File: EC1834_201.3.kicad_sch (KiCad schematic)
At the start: 72 parts

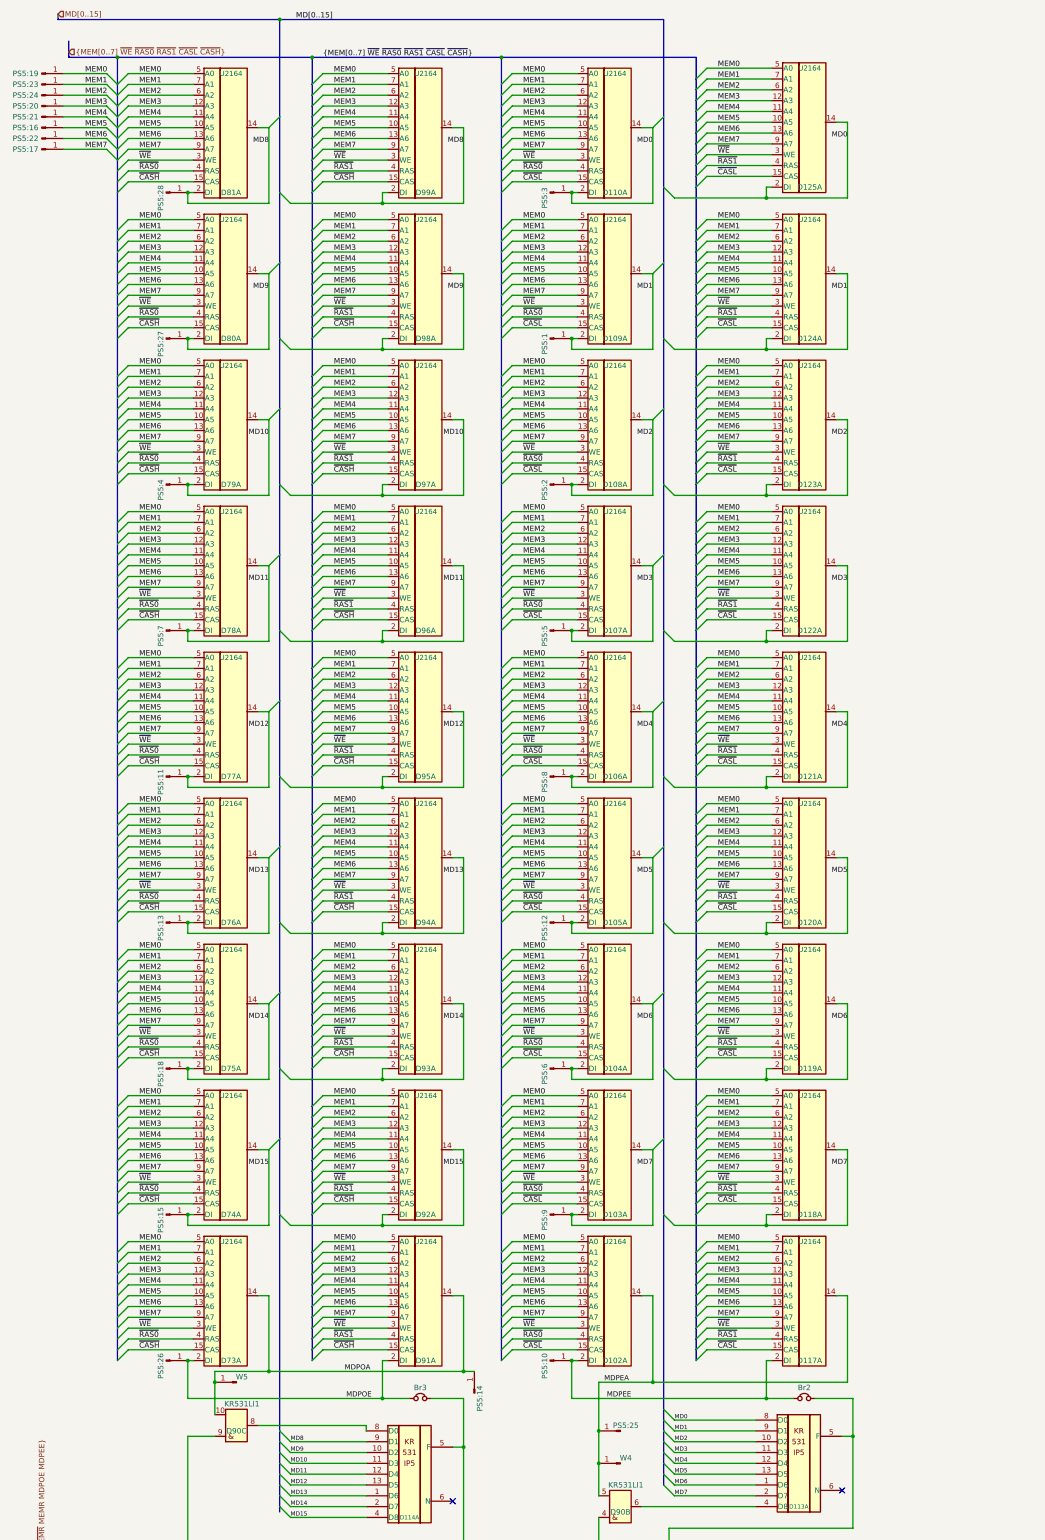
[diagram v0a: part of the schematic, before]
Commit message: Completed PCB layout Changed PS5
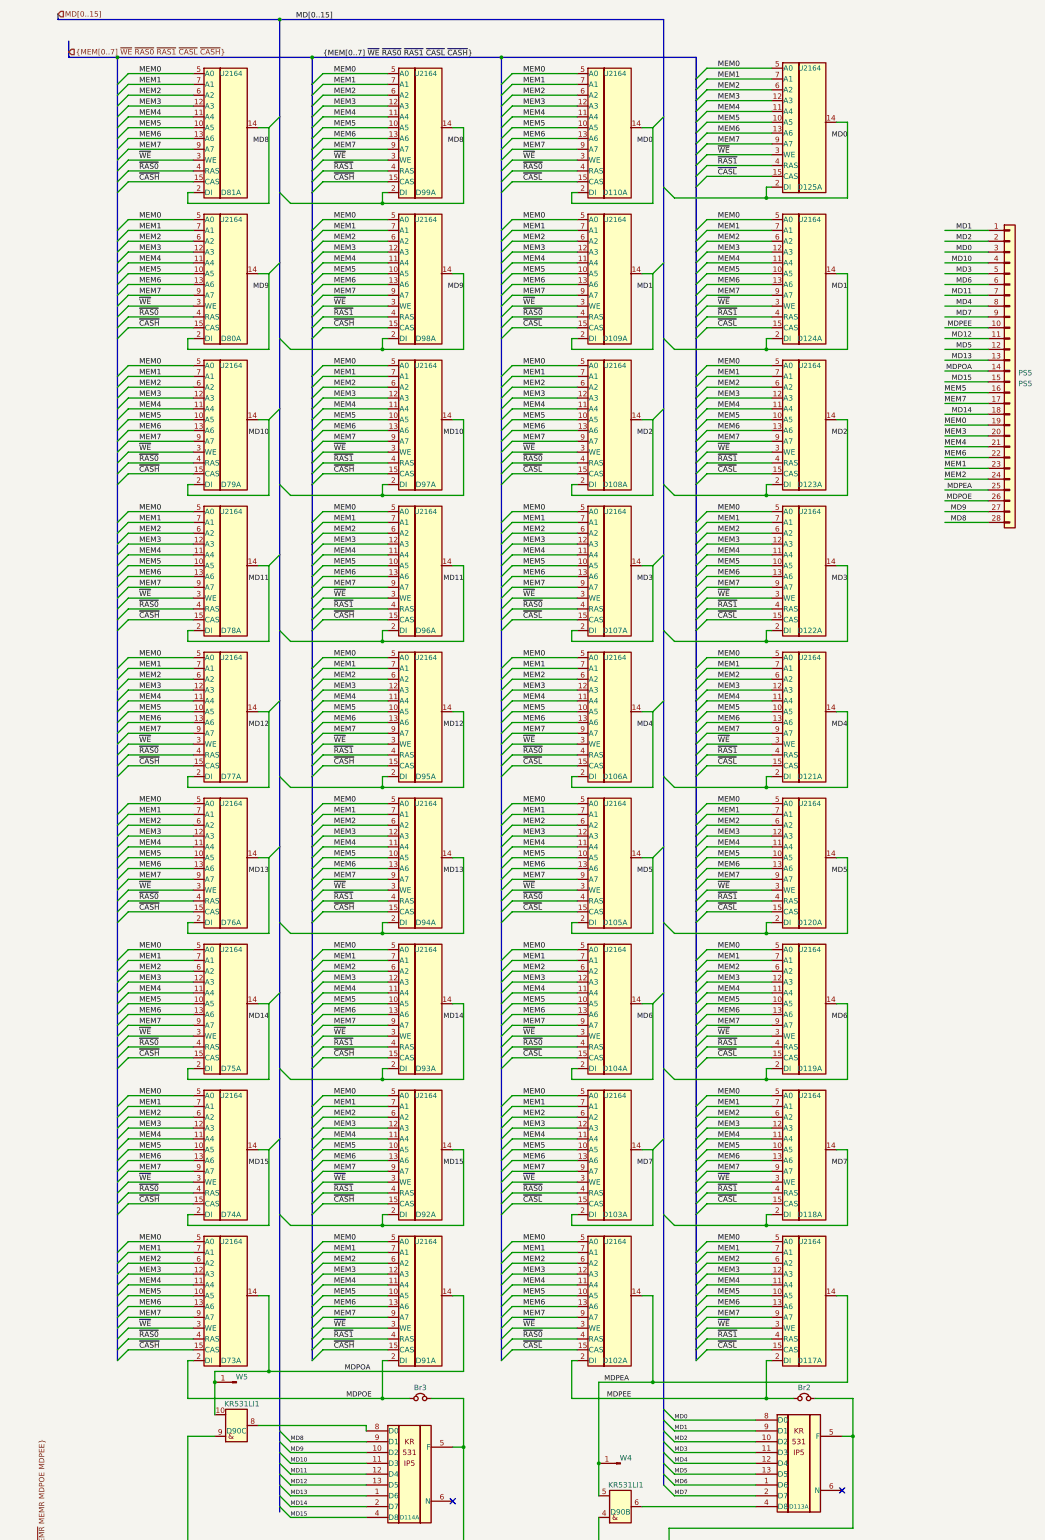
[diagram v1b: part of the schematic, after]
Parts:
- removed PS5:1, PS5:10, PS5:11, PS5:12, PS5:13, PS5:14, PS5:15, PS5:16, PS5:17, PS5:18, PS5:19, PS5:2, PS5:20, PS5:21, PS5:22, PS5:23, PS5:24, PS5:25, PS5:26, PS5:27, PS5:28, PS5:3, PS5:4, PS5:5, PS5:6, PS5:7, PS5:8, PS5:9: PS5, EC1834-Board:Pruefstecker5_Single, symbol Connector:Conn_01x01_Male
- added PS5: PS5, EC1834-Board:Pruefstecker5, symbol Connector_Generic:Conn_01x28
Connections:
- net MD0: now also PS5.3 (Pin_3)
- net MD1: now also PS5.1 (Pin_1)
- net MD10: now also PS5.4 (Pin_4)
- net MD11: now also PS5.7 (Pin_7)
- net MD12: now also PS5.11 (Pin_11)
- net MD13: now also PS5.13 (Pin_13)
- net MD14: now also PS5.18 (Pin_18)
- net MD15: now also PS5.15 (Pin_15)
- net MD2: now also PS5.2 (Pin_2)
- net MD3: now also PS5.5 (Pin_5)
- net MD4: now also PS5.8 (Pin_8)
- net MD5: now also PS5.12 (Pin_12)
- net MD6: now also PS5.6 (Pin_6)
- net MD7: now also PS5.9 (Pin_9)
- net MD8: now also PS5.28 (Pin_28)
- net MD9: now also PS5.27 (Pin_27)
- net MDPEA: now also PS5.25 (Pin_25)
- net MDPEE: now also PS5.10 (Pin_10)
- net MDPOA: now also PS5.14 (Pin_14)
- net MDPOE: now also PS5.26 (Pin_26)
- net MEM0: now also PS5.19 (Pin_19)
- net MEM1: now also PS5.23 (Pin_23)
- net MEM2: now also PS5.24 (Pin_24)
- net MEM3: now also PS5.20 (Pin_20)
- net MEM4: now also PS5.21 (Pin_21)
- net MEM5: now also PS5.16 (Pin_16)
- net MEM6: now also PS5.22 (Pin_22)
- net MEM7: now also PS5.17 (Pin_17)
